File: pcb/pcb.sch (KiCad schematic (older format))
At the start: 24 parts, among them J1 USB_B_Micro, J2 AVR ISP connector, J3 Display connector, J4 Conn_01x02_Male, SW1 SSSS811101, SW2 SW_DIP_x01, SW3 SW_DIP_x01, U1 ATmega328P-AU, U2 MCP73831-2-OT, U3 AP9101CK6, U4 DMN2053UVT, U5 DS3231MZ

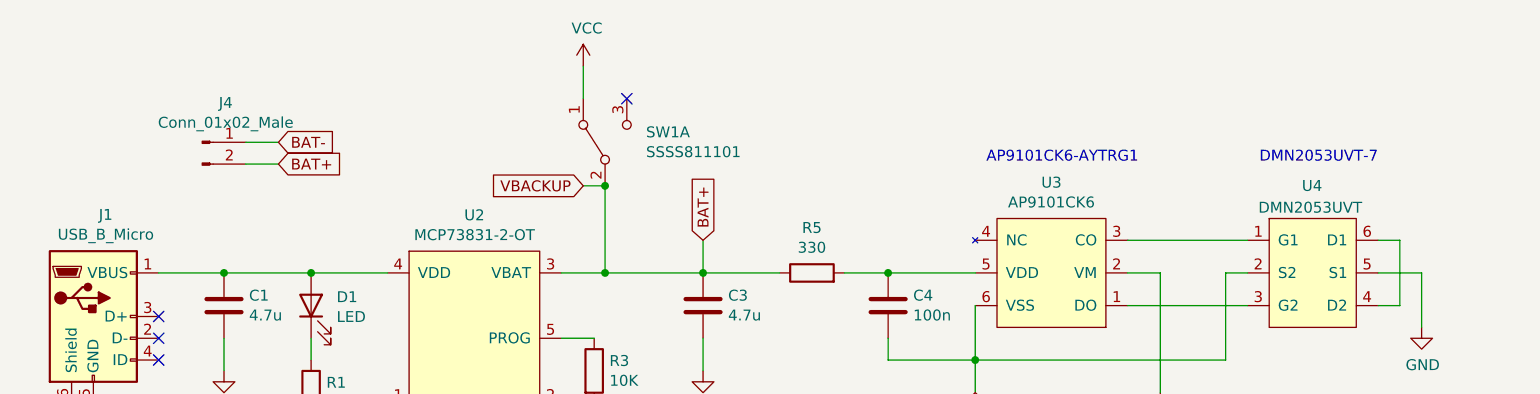
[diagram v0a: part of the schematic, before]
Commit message: Finalized schematic and PCB layout
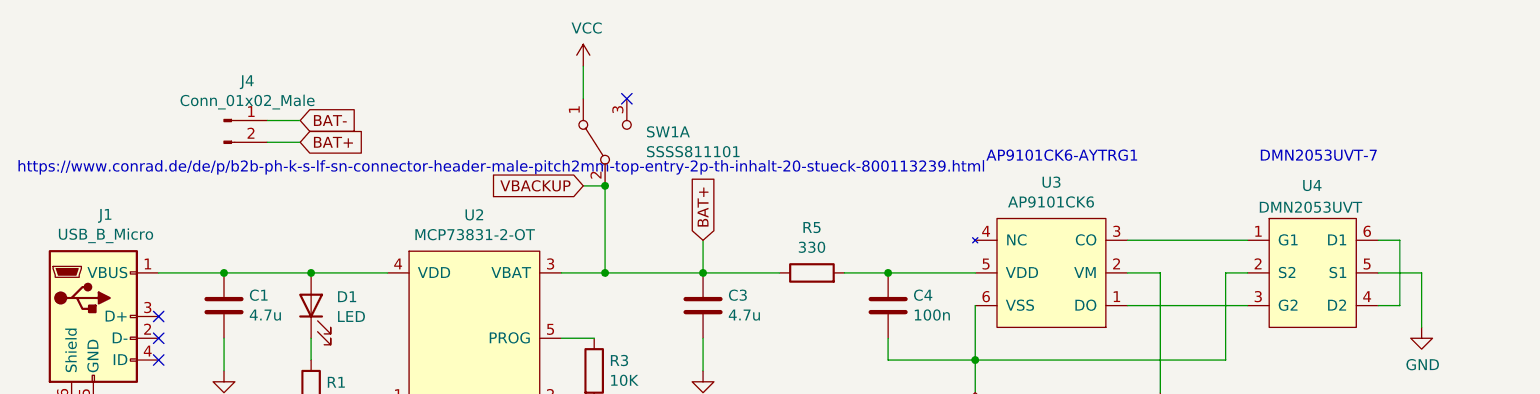
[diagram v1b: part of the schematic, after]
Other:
- note added: "https://www.conrad.de/de/p/b2b-ph-k-s-lf-sn-connector-header-male-pitch2mm-top-entry-2p-th-inhalt-20-stueck-800113239.html"
- moved on the sheet: J4
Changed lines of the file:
@@
 L Connector:Conn_01x02_Male J4
 U 1 1 5E792C70
-P 1700 1450
-F 0 "J4" H 1808 1631 50  0000 C CNN
-F 1 "Conn_01x02_Male" H 1808 1540 50  0000 C CNN
-F 2 "Connector_JST:JST_PH_B2B-PH-K_1x02_P2.00mm_Vertical" H 1700 1450 50  0001 C CNN
-F 3 "~" H 1700 1450 50  0001 C CNN
-	1    1700 1450
+P 1800 1350
+F 0 "J4" H 1908 1531 50  0000 C CNN
+F 1 "Conn_01x02_Male" H 1908 1440 50  0000 C CNN
+F 2 "Connector_JST:JST_PH_B2B-PH-K_1x02_P2.00mm_Vertical" H 1800 1350 50  0001 C CNN
+F 3 "~" H 1800 1350 50  0001 C CNN
+	1    1800 1350
 	1    0    0    -1
 $EndComp
-Text GLabel 2050 1550 2    50   Input ~ 0
+Text GLabel 2150 1450 2    50   Input ~ 0
 BAT+
-Text GLabel 2050 1450 2    50   Input ~ 0
+Text GLabel 2150 1350 2    50   Input ~ 0
 BAT-
 Wire Wire Line
-	2050 1450 1900 1450
+	2150 1350 2000 1350
 Wire Wire Line
-	1900 1550 2050 1550
+	2000 1450 2150 1450
 Wire Wire Line
 	6850 3850 7850 3850
@@
 Wire Wire Line
 	6850 3850 6850 3950
+Text Notes 850  1600 0    50   ~ 0
+https://www.conrad.de/de/p/b2b-ph-k-s-lf-sn-connector-header-male-pitch2mm-top-entry-2p-th-inhalt-20-stueck-800113239.html
 $EndSCHEMATC
